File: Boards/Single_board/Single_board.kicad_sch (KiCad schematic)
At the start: 9 parts, among them J1 AUX_I2C_1, J2 AUX_I2C_2, J4 ICSP, Q1 SI2306

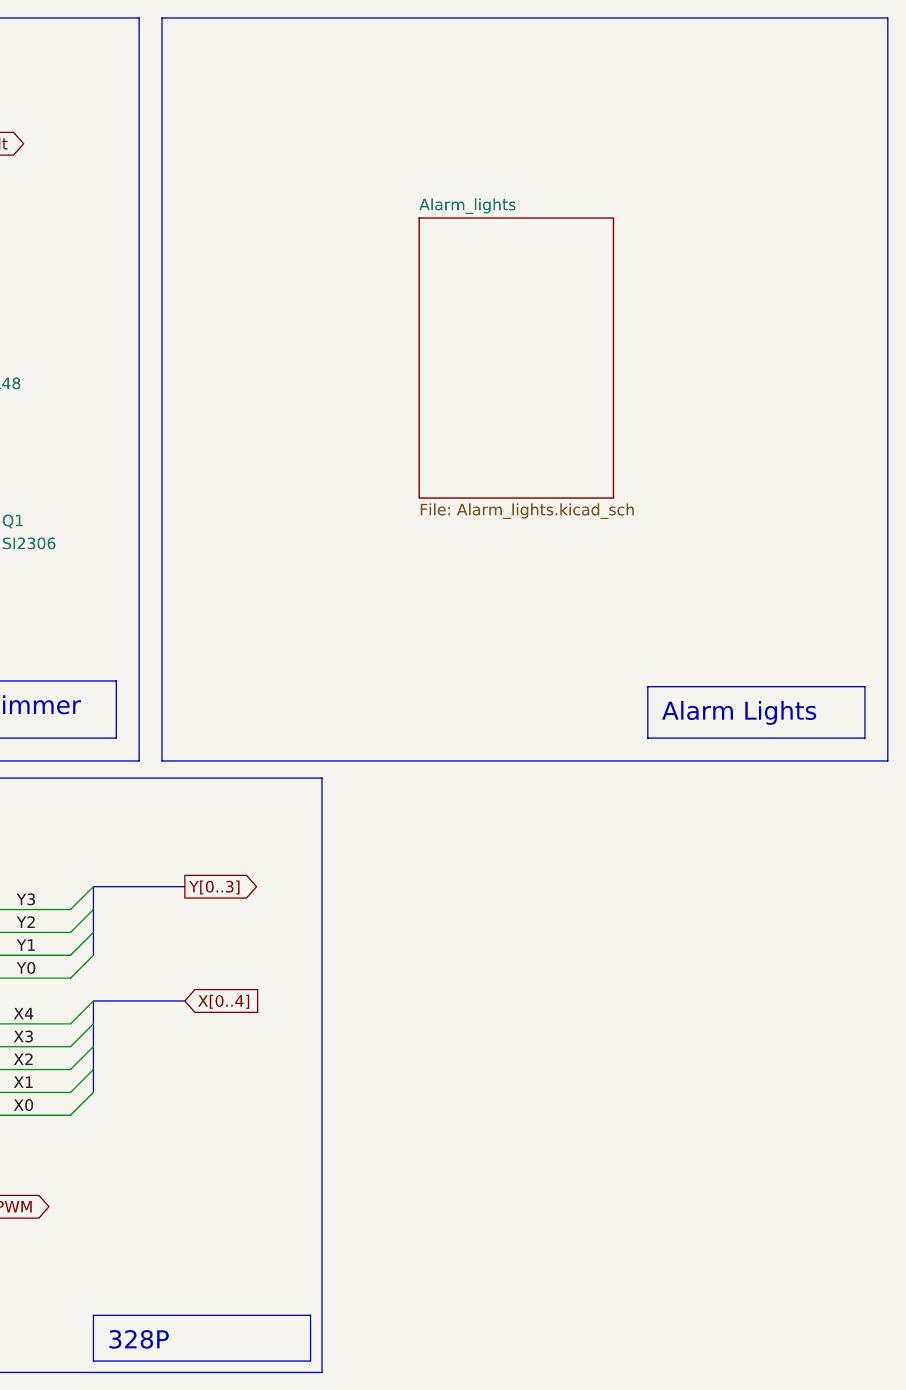
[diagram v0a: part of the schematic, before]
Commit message: Fixes on single board
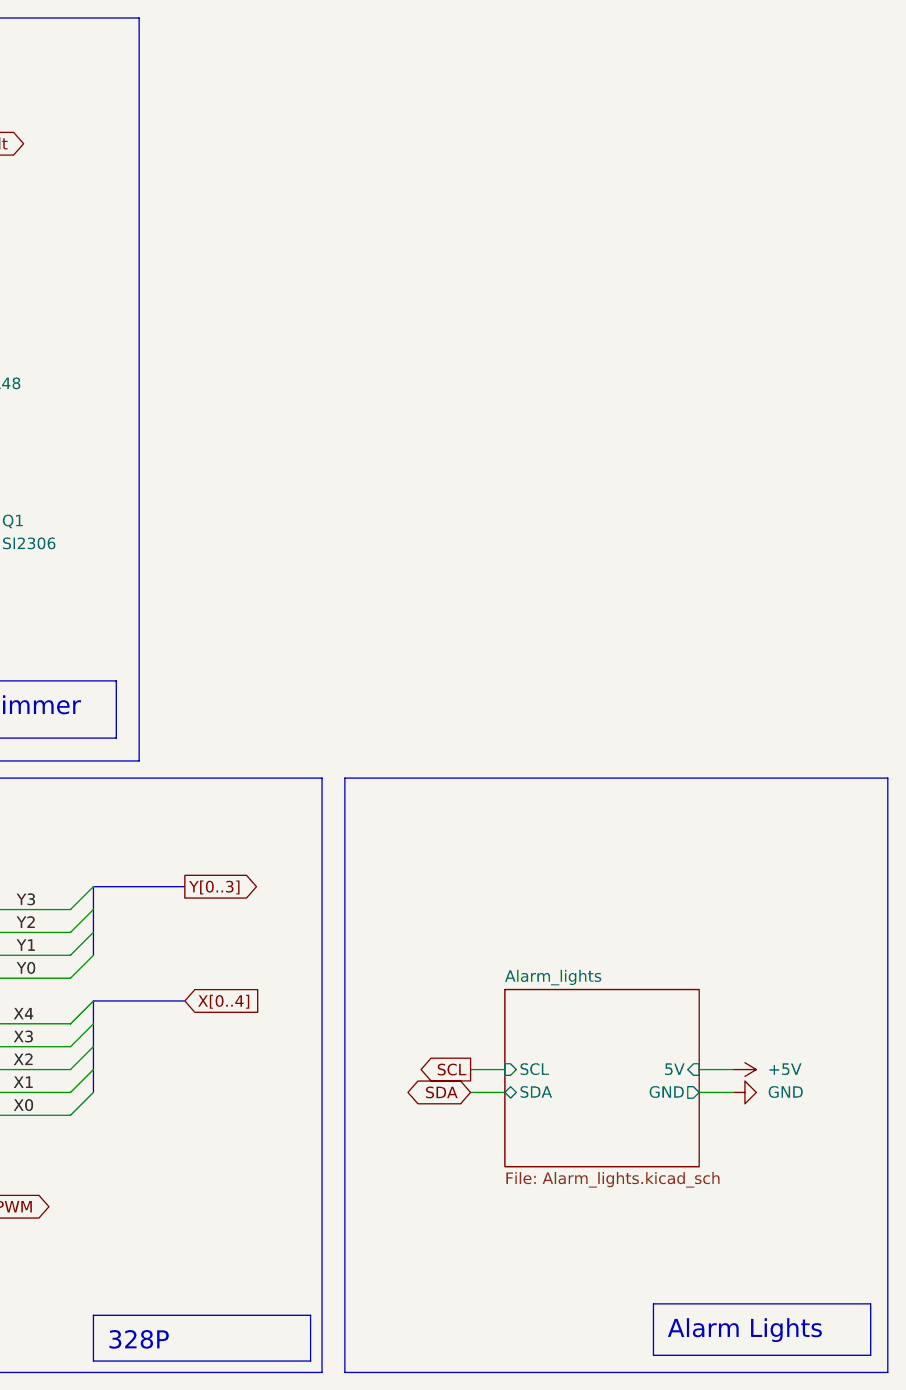
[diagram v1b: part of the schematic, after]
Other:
- sheet Alarm_lights ports: added 5V, GND, SCL, SDA; removed none
